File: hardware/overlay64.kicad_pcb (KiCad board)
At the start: 2 copper layers, 31.8 x 35.6 mm, 17 parts, among them IC1 ATMEGA328P-P, P1 ISP, P2 MAIN, P3 INPUT/BYPASS, Q1 BC547B, U1 LM1881, Y1 20MHz

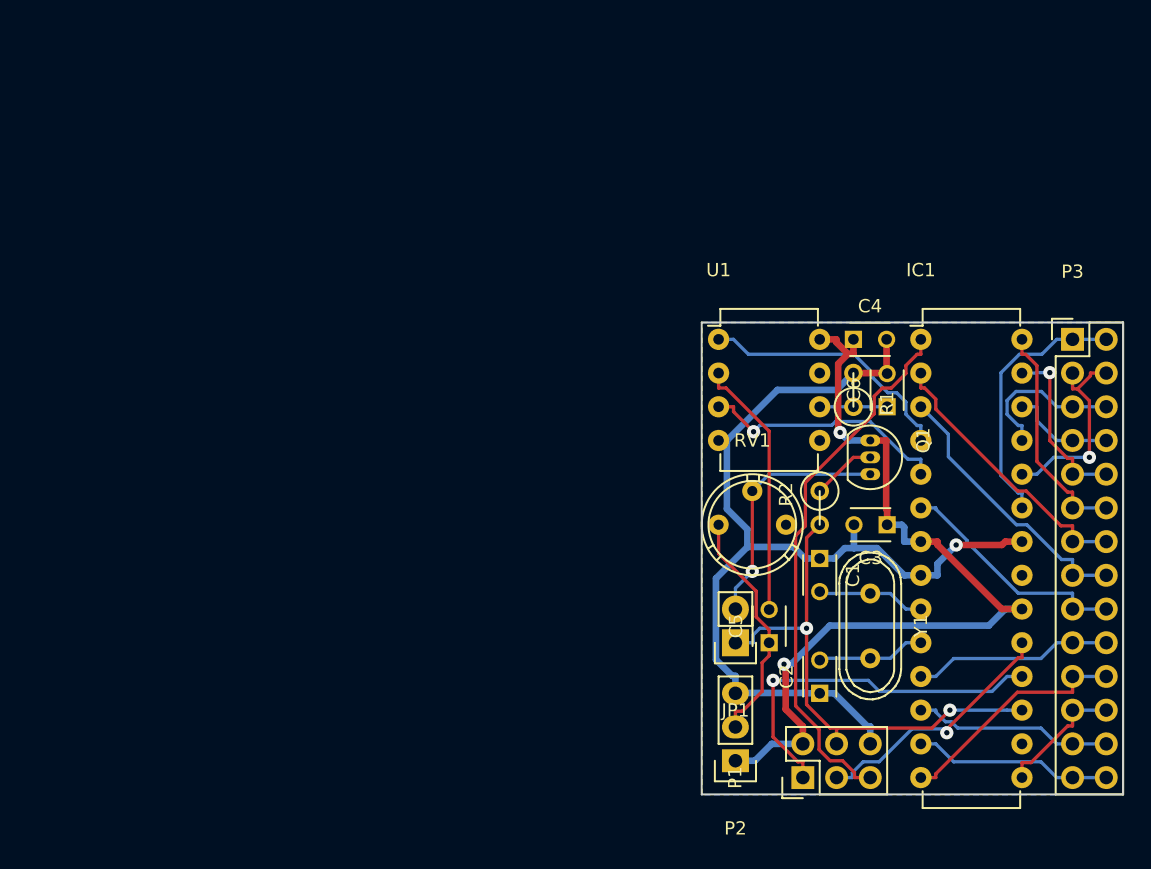
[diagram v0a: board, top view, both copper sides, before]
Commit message: Hardware: Rearranged components, rerouting...
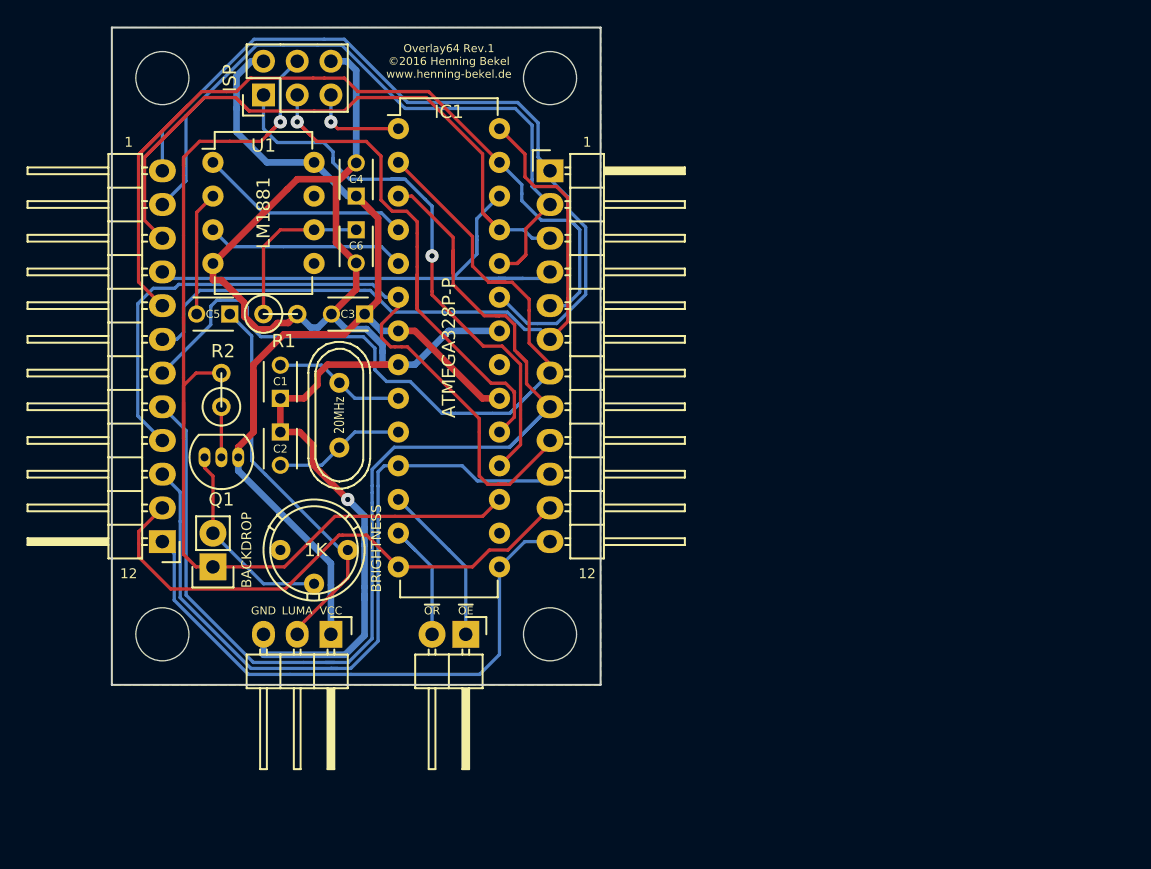
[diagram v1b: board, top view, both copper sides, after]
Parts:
- removed RV1: 1k, Potentiometers:Potentiometer_Bourns_3339P_Angular_ScrewUp
- added 1K: 1k, Potentiometers:Potentiometer_Bourns_3339P_Angular_ScrewUp, F.Cu at (100.3, 95.2)
- added H1: MountingHole_4mm, Mounting_Holes:MountingHole_4mm, F.Cu at (86.4, 59.7)
- added H2: MountingHole_4mm, Mounting_Holes:MountingHole_4mm, F.Cu at (115.6, 59.7)
- added H3: MountingHole_4mm, Mounting_Holes:MountingHole_4mm, F.Cu at (86.4, 101.6)
- added H4: MountingHole_4mm, Mounting_Holes:MountingHole_4mm, F.Cu at (115.6, 101.6)
- added P4: BYPASS, Pin_Headers:Pin_Header_Angled_1x12, F.Cu at (115.6, 66.7)
- added P5: INPUT, Pin_Headers:Pin_Header_Angled_1x12, F.Cu at (86.4, 94.6)
- P2: footprint Pin_Headers:Pin_Header_Straight_1x03 -> Pin_Headers:Pin_Header_Angled_1x03
- P3: value INPUT/BYPASS -> CONTROL; footprint Pin_Headers:Pin_Header_Straight_2x14 -> Pin_Headers:Pin_Header_Angled_1x02
- moved P1 65.6 mm to (94.0, 61.0)
- moved P3 50.8 mm to (109.2, 101.6), turned to 270 degrees
- moved Q1 47.6 mm to (92.1, 88.3), turned to 180 degrees
- moved C5 47.6 mm to (91.4, 77.5), turned to 180 degrees
- moved R2 46.0 mm to (90.8, 83.2), turned to 90 degrees
- moved C2 45.2 mm to (95.2, 86.4), turned to 270 degrees
- moved R1 43.6 mm to (95.2, 77.5), turned to 0 degrees
- moved Y1 43.0 mm to (99.7, 85.1)
- moved C3 42.5 mm to (101.6, 77.5)
- moved IC1 42.5 mm to (104.1, 63.5)
- moved C1 42.4 mm to (95.2, 83.8), turned to 90 degrees
- moved C6 42.2 mm to (101.0, 71.1), turned to 270 degrees
- moved U1 40.4 mm to (90.2, 66.0)
- moved JP1 39.8 mm to (90.2, 96.5)
- moved C4 39.0 mm to (101.0, 68.6), turned to 90 degrees
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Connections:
- P3 pad 1: /IN0 -> /~OE
- P3 pad 2: /IN0 -> /~OR
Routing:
- net /IN7: track 20.9 -> 91.3 mm
- net /IN4: track 13.2 -> 66.8 mm, vias 1 -> 0
- net /IN6: track 21.0 -> 67.6 mm
- net /MOSI: track 38.8 -> 82.5 mm, vias 2 -> 1
- net /IN2: track 11.9 -> 54.9 mm
- net /IN8: track 17.9 -> 57.9 mm
- net /IN9: track 15.0 -> 54.9 mm
- net /IN0: track 20.0 -> 59.4 mm
- net /IN1: track 15.5 -> 53.1 mm, vias 1 -> 0
- net /IN5: track 17.2 -> 53.6 mm
- net /IN3: track 8.01 -> 42.0 mm
- net /~RESET: track 41.1 -> 7.32 mm, vias 0 -> 1
- net /IN11: track 9.81 -> 43.4 mm
- net GND: track 76.8 -> 108.3 mm
- net /IN10: track 18.0 -> 41.2 mm
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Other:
- board size 31.8 x 35.6 mm -> 36.8 x 49.5 mm
- board text added: "1"
- board text added: "12"
- board text added: "20MHz"
- board text added: "BACKDROP"
- board text added: "BRIGHTNESS"
- board text added: "C1"
- board text added: "C2"
- board text added: "C3"
- board text added: "C4"
- board text added: "C5"
- board text added: "C6"
- board text added: "GND"
- board text added: "LUMA"
- board text added: "Overlay64 Rev.1 ©2016 Henning Bekel www.henning-bekel.de"
- board text added: "VCC"
- board text added: "~OE"
- board text added: "~OR"
